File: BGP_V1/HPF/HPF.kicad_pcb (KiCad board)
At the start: 2 copper layers, 30 x 30 mm, 12 parts, among them P1 CONN_01X05, U1 OPA2170

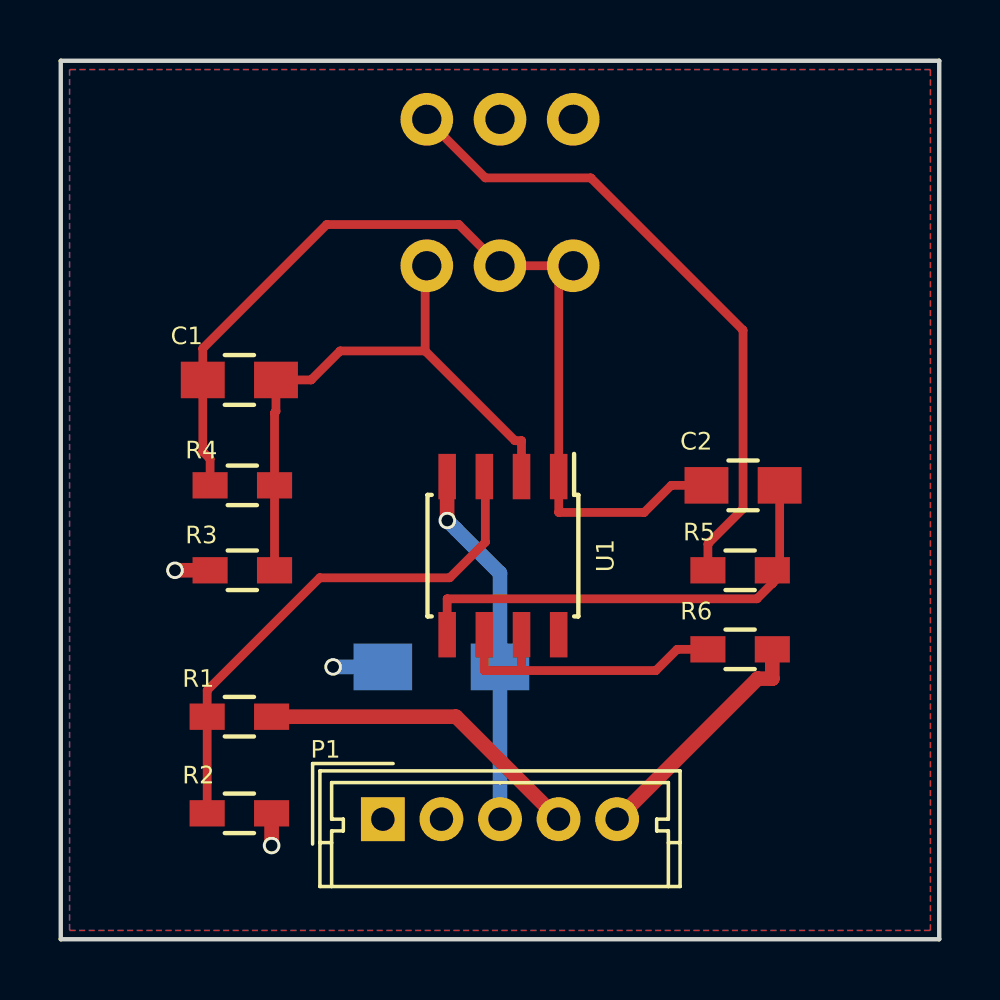
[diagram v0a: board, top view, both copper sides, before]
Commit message: BOM for V1 BGP
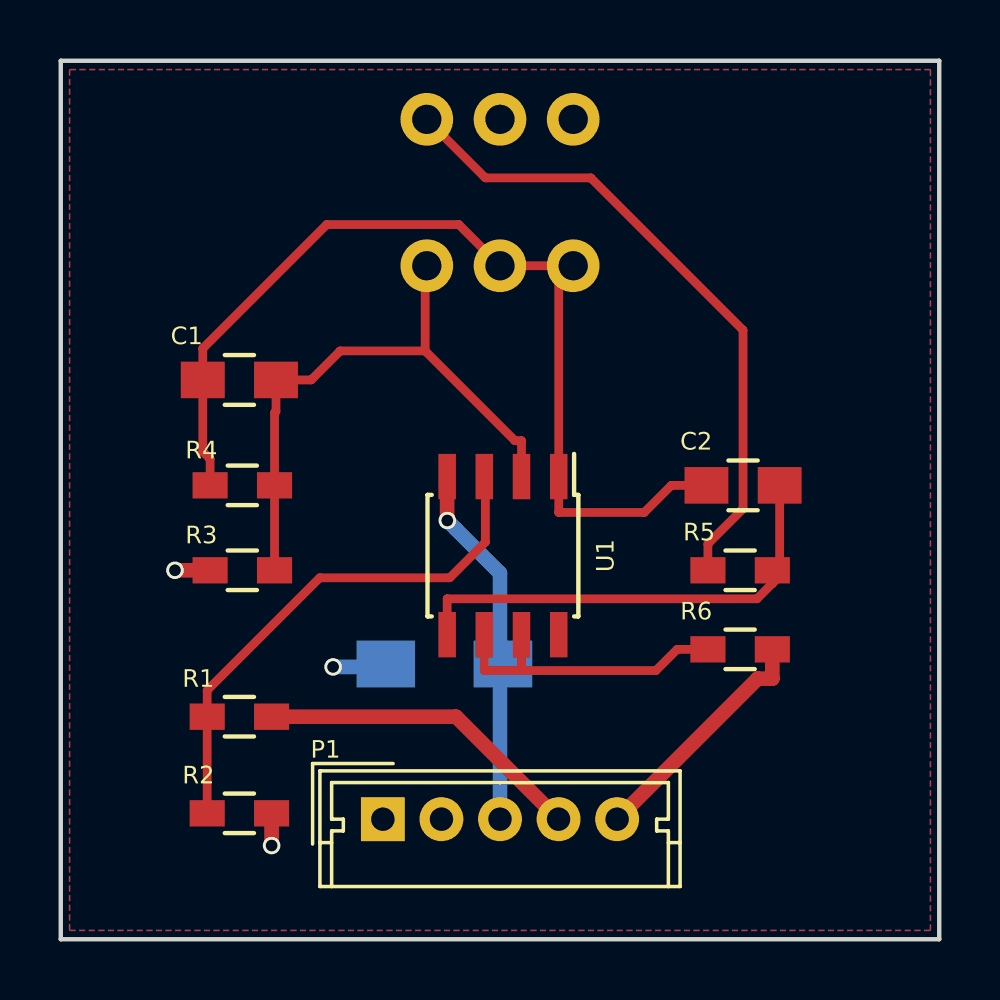
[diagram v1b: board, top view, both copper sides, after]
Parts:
- moved C3 0.14 mm to (153.1, 70.6)
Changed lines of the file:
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@@
   (page A4)
   (layers
-    (0 F.Cu signal)
+    (0 F.Cu signal hide)
     (31 B.Cu signal)
     (32 B.Adhes user)
@@
     )
   )
-  (module Capacitors_SMD:C_1206_HandSoldering (layer B.Cu)
-    (at 153 70.7)
-    (descr "Capacitor SMD 1206, hand soldering")
-    (tags "capacitor 1206")
-    (attr smd)
-    (fp_text reference C3 (at 2.6 -1.6) (layer B.SilkS)
-      (effects (font (size 0.6 0.6) (thickness 0.15)) (justify mirror))
-    )
-    (fp_text value 10u (at 0 -2.3) (layer B.Fab) hide
-      (effects (font (size 0.6 0.6) (thickness 0.15)) (justify mirror))
-    )
-    (fp_line (start -3.3 1.15) (end 3.3 1.15) (layer B.CrtYd) (width 0.05))
-    (fp_line (start -3.3 -1.15) (end 3.3 -1.15) (layer B.CrtYd) (width 0.05))
-    (fp_line (start -3.3 1.15) (end -3.3 -1.15) (layer B.CrtYd) (width 0.05))
-    (fp_line (start 3.3 1.15) (end 3.3 -1.15) (layer B.CrtYd) (width 0.05))
-    (fp_line (start 1 1.025) (end -1 1.025) (layer B.SilkS) (width 0.15))
-    (fp_line (start -1 -1.025) (end 1 -1.025) (layer B.SilkS) (width 0.15))
-    (pad 1 smd rect (at -2 0) (size 2 1.6) (layers B.Cu B.Paste B.Mask)
-      (net 4 /V+))
-    (pad 2 smd rect (at 2 0) (size 2 1.6) (layers B.Cu B.Paste B.Mask)
-      (net 5 /V-))
-    (model Capacitors_SMD.3dshapes/C_1206_HandSoldering.wrl
-      (at (xyz 0 0 0))
-      (scale (xyz 1 1 1))
-      (rotate (xyz 0 0 0))
-    )
-  )
   (module Resistors_SMD:R_0603_HandSoldering (layer F.Cu)
     (at 146.1 72.4)
@@
       (rotate (xyz 0 0 0))
     )
+  )
+  (module Capacitors_SMD:C_1206_HandSoldering (layer B.Cu)
+    (at 153.1 70.6)
+    (descr "Capacitor SMD 1206, hand soldering")
+    (tags "capacitor 1206")
+    (attr smd)
+    (fp_text reference C3 (at 2.8 -1.6) (layer B.SilkS)
+      (effects (font (size 0.6 0.6) (thickness 0.15)) (justify mirror))
+    )
+    (fp_text value 10u (at 0 -2.3) (layer B.Fab) hide
+      (effects (font (size 0.6 0.6) (thickness 0.15)) (justify mirror))
+    )
+    (fp_line (start -3.3 1.15) (end 3.3 1.15) (layer B.CrtYd) (width 0.05))
+    (fp_line (start -3.3 -1.15) (end 3.3 -1.15) (layer B.CrtYd) (width 0.05))
+    (fp_line (start -3.3 1.15) (end -3.3 -1.15) (layer B.CrtYd) (width 0.05))
+    (fp_line (start 3.3 1.15) (end 3.3 -1.15) (layer B.CrtYd) (width 0.05))
+    (fp_line (start 1 1.025) (end -1 1.025) (layer B.SilkS) (width 0.15))
+    (fp_line (start -1 -1.025) (end 1 -1.025) (layer B.SilkS) (width 0.15))
+    (pad 1 smd rect (at -2 0) (size 2 1.6) (layers B.Cu B.Paste B.Mask)
+      (net 4 /V+))
+    (pad 2 smd rect (at 2 0) (size 2 1.6) (layers B.Cu B.Paste B.Mask)
+      (net 5 /V-))
+    (model Capacitors_SMD.3dshapes/C_1206_HandSoldering.wrl
+      (at (xyz 0 0 0))
+      (scale (xyz 1 1 1))
+      (rotate (xyz 0 0 0))
+    )
